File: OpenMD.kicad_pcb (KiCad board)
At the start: 4 copper layers, 90 x 55 mm, 189 parts, among them IC1 MP9485GN-Z, J1 GND, J2 Digital, J3 Analog, J4 Sensors, J5 A, J6 B, J7 C, J8 V_{BATT}, Q1 EPC2088, Q2 EPC2088, Q3 EPC2088, Q7 EPC2088, Q8 EPC2088, Q9 EPC2088, U1 UP1966E, U10 INA241A2xDDF, U2 UP1966E, U3 UP1966E, U7 ADA4610-4xCP, U8 INA241A2xDDF, U9 INA241A2xDDF

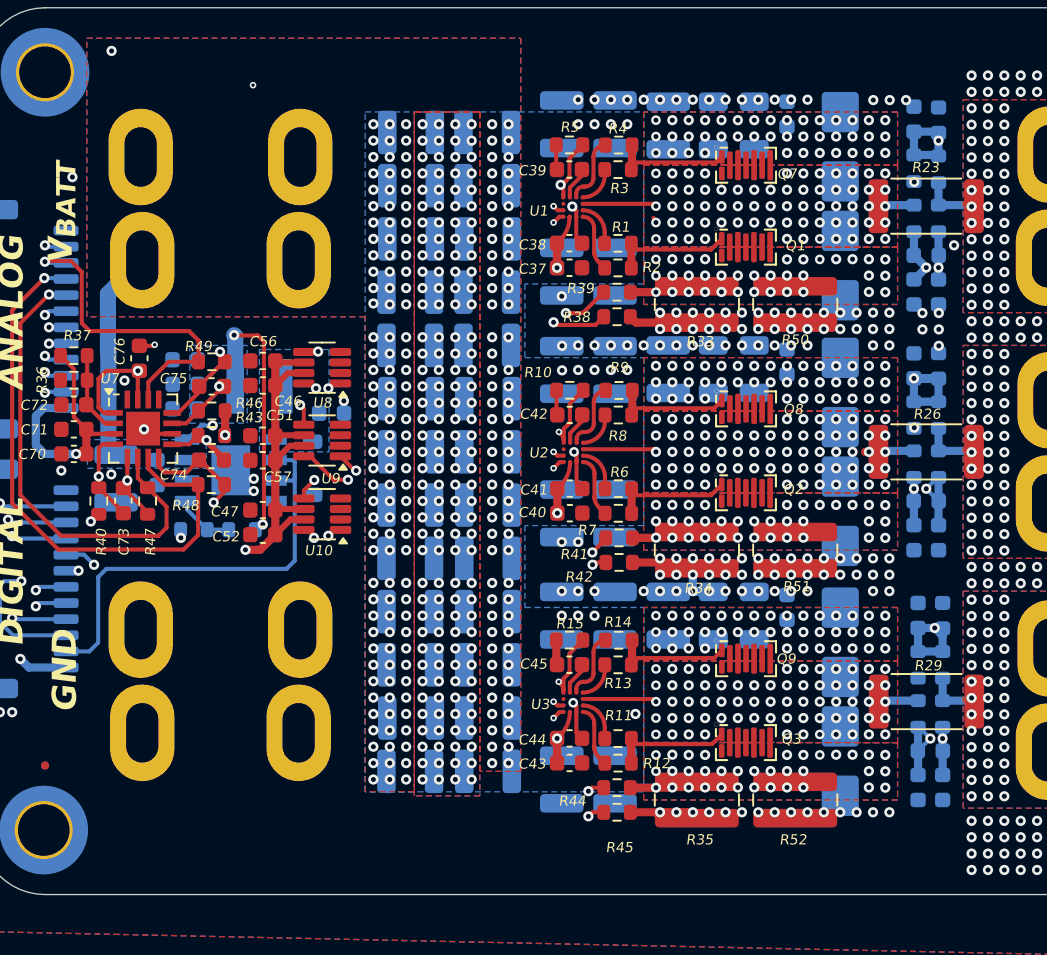
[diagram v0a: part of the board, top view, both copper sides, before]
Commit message: added license and almost ready for prod
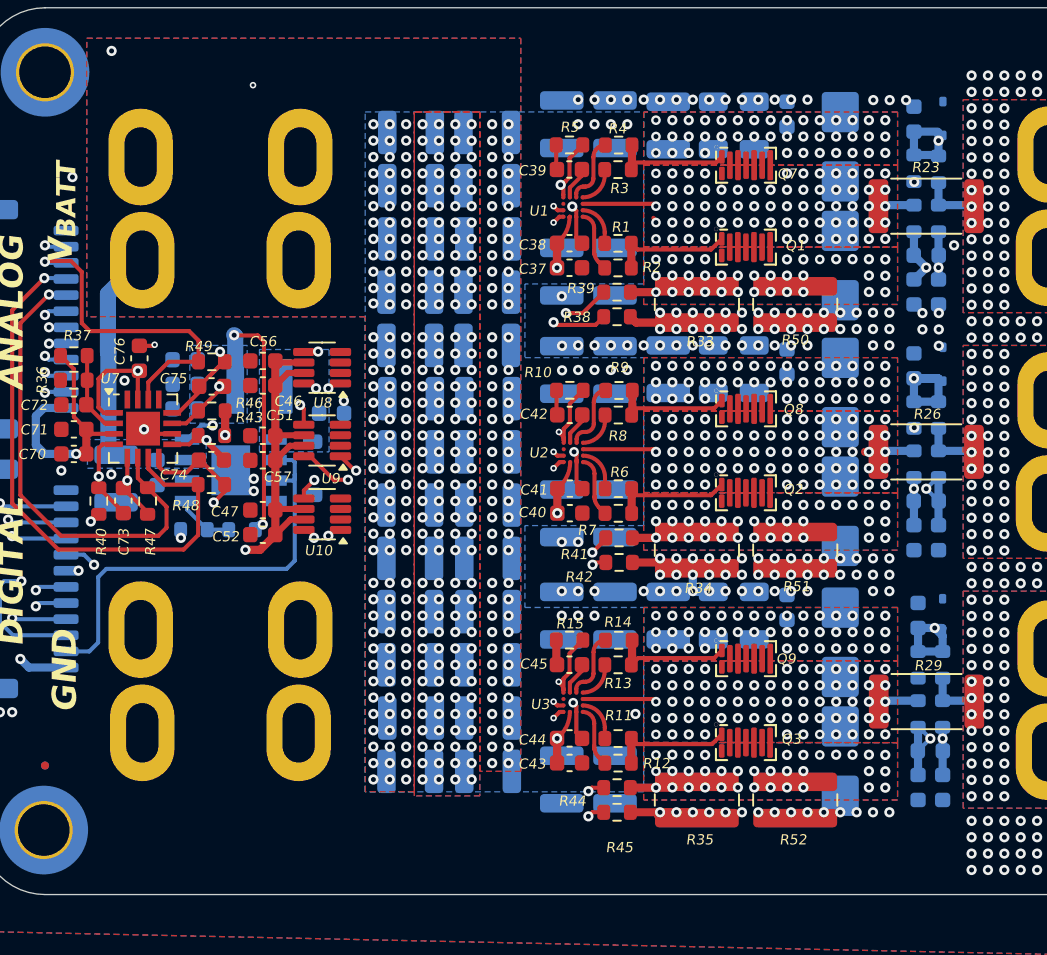
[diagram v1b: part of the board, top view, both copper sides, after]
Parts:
- removed REF**: ESD-Logo_6.6x6mm_SilkScreen, Symbol:ESD-Logo_6.6x6mm_SilkScreen
- removed REF**: OSHW-Symbol_6.7x6mm_SilkScreen, Symbol:OSHW-Symbol_6.7x6mm_SilkScreen
- removed REF**: WEEE-Logo_4.2x6mm_SilkScreen, Symbol:WEEE-Logo_4.2x6mm_SilkScreen
- D10: value D_Schottky -> 1V
- D7, D8, D9: footprint Diode_SMD:D_0603_1608Metric -> Diode_SMD:D_SOD-323
- moved D7 0.29 mm to (152.8, 82.2)
- moved D8 0.29 mm to (152.8, 97.4)

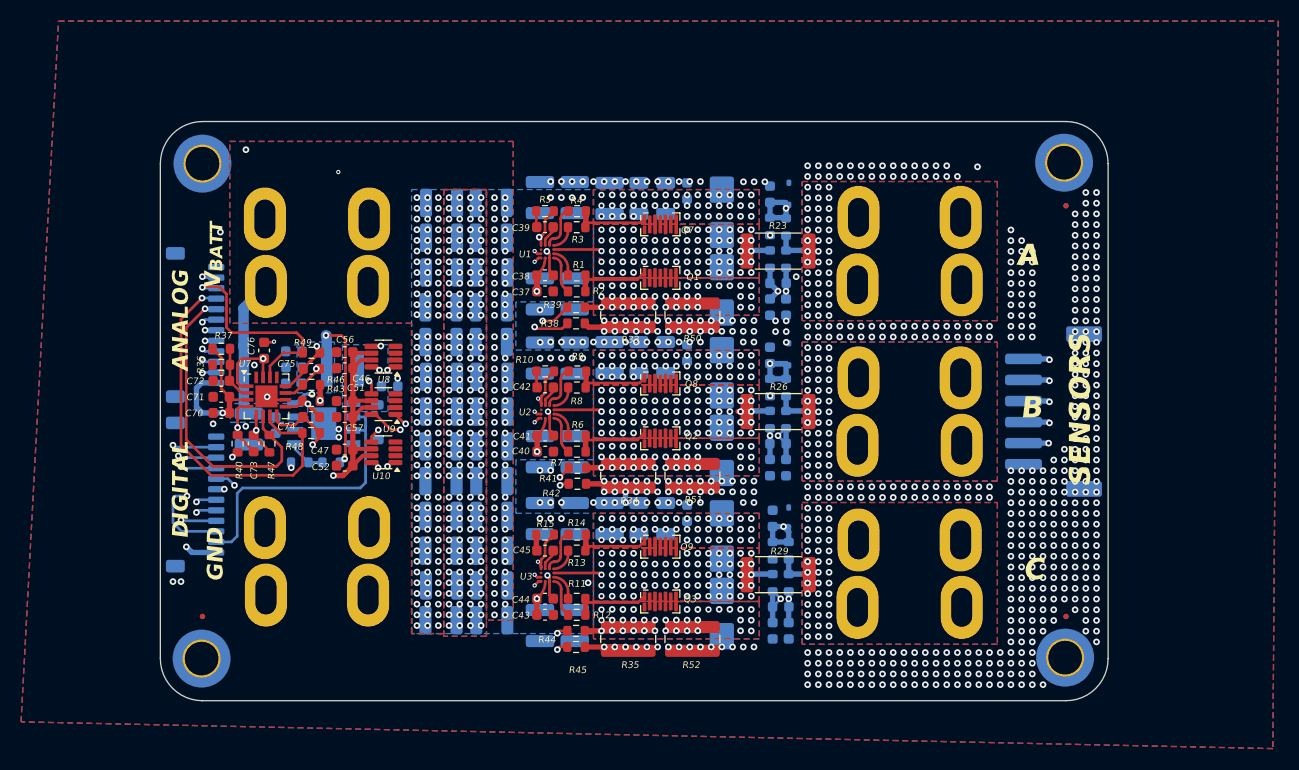
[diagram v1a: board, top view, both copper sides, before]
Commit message: first fab run
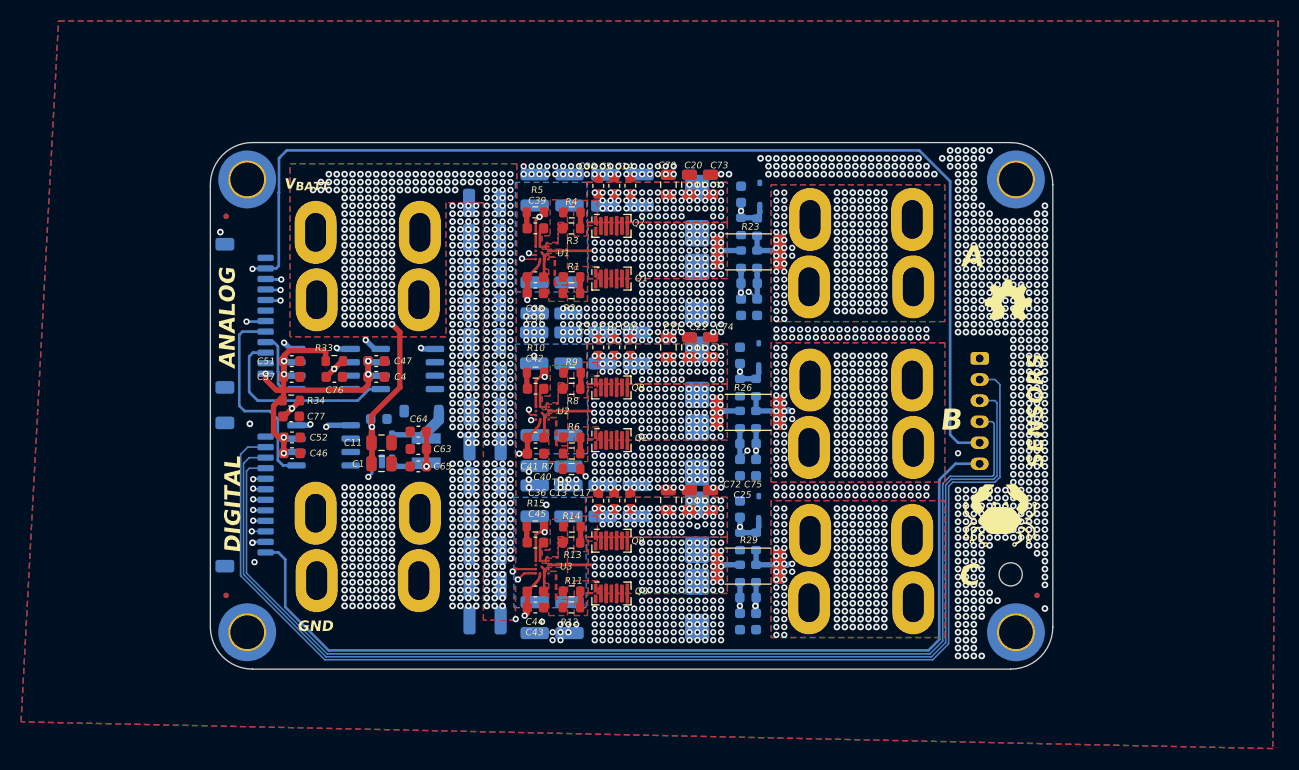
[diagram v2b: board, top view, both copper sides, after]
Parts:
- removed C56: 4.7uF, Capacitor_SMD:C_0603_1608Metric
- removed C61, C83, C84, C85: 10uF, Capacitor_SMD:C_1210_3225Metric
- removed C66: 100nF, Capacitor_SMD:C_0603_1608Metric
- removed the G*** at (139.1, 105.6)
- removed IC1: MP9485GN-Z, OpenMD:SOIC127P600X170-9N
- removed R31, R32: 240k, Resistor_SMD:R_0603_1608Metric
- removed R35, R50, R51, R52: .5m, Resistor_SMD:R_1020_2550Metric
- removed R36, R37, R40, R43, R46, R47, R48, R49: 20k, Resistor_SMD:R_0603_1608Metric
- removed R38, R39, R41, R42, R44, R45: 1k, Resistor_SMD:R_0603_1608Metric
- removed U7: ADA4610-4xCP, Package_CSP:LFCSP-16-1EP_4x4mm_P0.65mm_EP2.1x2.1mm
- added G***: LOGO, OpenMD:CrabLabs, F.Cu at (172.9, 112.7)
- added G***: LOGO, OpenMD:CrabLabs, B.Cu at (172.9, 88.1)
- added H6: M2, MountingHole:MountingHole_2.2mm_M2, F.Cu at (173.9, 118.3)
- added IC2: RAA2118054GP3#JA0, Package_TO_SOT_SMD:SOT-23-5, B.Cu at (114.2, 106.5)
- added SYM1: Logo_Open_Hardware_Large, Symbol:OSHW-Symbol_8.9x8mm_SilkScreen, F.Cu at (173.6, 92.3)
- added SYM1: Logo_Open_Hardware_Large, Symbol:OSHW-Symbol_8.9x8mm_SilkScreen, B.Cu at (173.6, 113.8)
- added TH1: 10k, Resistor_SMD:R_0603_1608Metric, F.Cu at (132.2, 108.3)
- C1, C11, C20, C22, C25: value 10uF -> 1uF; footprint Capacitor_SMD:C_1210_3225Metric -> Capacitor_SMD:C_0805_2012Metric; moved to F.Cu
- C10, C13, C14, C16, C17, C5, C77: value 10uF -> 100nF; footprint Capacitor_SMD:C_1210_3225Metric -> Capacitor_SMD:C_0603_1608Metric; moved to F.Cu
- C12, C15, C18, C19, C2, C21, C23, C24, C26, C27, C3, C6, C7, C78, C79, C8, C80, C81, C82, C86, C87, C88, C89, C9, C91: value 10uF -> 4.7uF
- C28, C29, C31, C32, C34, C35: footprint Capacitor_SMD:C_1206_3216Metric -> Capacitor_SMD:C_1210_3225Metric
- C30, C33, C36, C63, C64, C65: moved to F.Cu
- C4: value 10uF -> 4.7uF; footprint Capacitor_SMD:C_1210_3225Metric -> Capacitor_SMD:C_0603_1608Metric; moved to F.Cu
- C70: value 100nF -> 1uF; footprint Capacitor_SMD:C_0603_1608Metric -> Capacitor_SMD:C_0805_2012Metric
- C71: value 4.7uF -> 1uF; footprint Capacitor_SMD:C_0603_1608Metric -> Capacitor_SMD:C_0805_2012Metric
- C72, C73, C74, C75: value 10nF -> 1uF; footprint Capacitor_SMD:C_0603_1608Metric -> Capacitor_SMD:C_0805_2012Metric
- D1, D2, D3, D4, D5, D6: value S3BB-13-F -> .85V
- D10: value 1V -> .85V
- D7, D8, D9: value 3.7V -> 3.3V
- H1, H2, H3, H4: value MountingHole_Pad -> M3
- J4: footprint Connector_JST:JST_PH_S6B-PH-SM4-TB_1x06-1MP_P2.00mm_Horizontal -> Connector_JST:JST_PH_S6B-PH-K_1x06_P2.00mm_Horizontal
- L1: value 33uH -> 22uH; footprint Inductor_SMD:L_Abracon_ASPI-4030S -> Inductor_SMD:L_Abracon_ASPI-3012S
- Q1, Q2, Q3, Q7, Q8, Q9: value EPC2088 -> EPC2065
- R1, R11, R14, R4, R6, R9: value 0 -> 1
- R33, R34: value .5m -> 10k; footprint Resistor_SMD:R_1020_2550Metric -> Resistor_SMD:R_0603_1608Metric
- U10, U8, U9: value INA241A2xDDF -> INA240A2; footprint Package_TO_SOT_SMD:SOT-23-8 -> Package_SO:SO-8_3.9x4.9mm_P1.27mm; moved to B.Cu
- moved FID2 79.8 mm to (99.4, 84.3)
- moved FID6 79.8 mm to (99.4, 84.3)
- moved C73 49.9 mm to (145.4, 81.3)
- moved C70 47.7 mm to (141.4, 81.3), turned to 90 degrees
- moved C20 47.6 mm to (143.4, 81.3), turned to 90 degrees
- moved C72 43.9 mm to (141.4, 111.3), turned to 90 degrees
- moved C71 42.7 mm to (141.4, 96.8), turned to 90 degrees
- moved C75 39.9 mm to (145.4, 111.3), turned to 90 degrees
- moved C74 38.5 mm to (145.4, 96.8), turned to 90 degrees
- moved C14 33.3 mm to (137.8, 81.4), turned to 90 degrees
- moved R34 32.8 mm to (105.6, 101.8), turned to 0 degrees
- moved C11 31.7 mm to (114.1, 105.8), turned to 0 degrees
- moved C22 28.5 mm to (143.4, 96.8), turned to 90 degrees
- moved R33 28.2 mm to (109.7, 98.1), turned to 0 degrees
- moved C13 27.2 mm to (136.3, 111.3), turned to 90 degrees
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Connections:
- C4 pad 1: /V_{BATT} -> /V_{ANA}
- C70 pad 1: /V_{ANA} -> /V_{BATT}
- C71 pad 1: /V_{ANA} -> /V_{BATT}
- C72 pad 1: Net-(U7A-+) -> /V_{BATT}
- C73 pad 1: Net-(U7B-+) -> /V_{BATT}
- C73 pad 2: Net-(U7B--) -> /GND
- C74 pad 1: Net-(U7C-+) -> /V_{BATT}
- C74 pad 2: Net-(U7C--) -> /GND
- C75 pad 1: Net-(U7D-+) -> /V_{BATT}
- C75 pad 2: Net-(U7D--) -> /GND
- C76 pad 1: /Driver Current Sensors/V_{REF} -> /M_TEMP_SENSE
- C77 pad 1: /V_{BATT} -> /DRV_TEMP_SENSE
- J3 pad 10: /DRV_I_SENSE.C -> /V_SENSE.C
- J3 pad 2: /I_SENSE.A -> /GND
- J3 pad 3: /I_SENSE.B -> /I_SENSE.A
- J3 pad 4: /I_SENSE.C -> /I_SENSE.B
- J3 pad 5: /V_SENSE.A -> /I_SENSE.C
- J3 pad 6: /V_SENSE.B -> /DRV_TEMP_SENSE
- J3 pad 7: /V_SENSE.C -> /GND
- J3 pad 8: /DRV_I_SENSE.A -> /V_SENSE.A
- J3 pad 9: /DRV_I_SENSE.B -> /V_SENSE.B
- J4 pad 1: /V_{DIG} -> /GND
- J4 pad 2: /M_TEMP_SENSE -> /HALL.C
- J4 pad 3: /HALL.A -> /HALL.B
- J4 pad 4: /HALL.B -> /HALL.A
- J4 pad 5: /HALL.C -> /M_TEMP_SENSE
- J4 pad 6: /GND -> /V_{DIG}
- Q1 pad 2: /DRV_CURR_SENSE.A -> /GND
- Q1 pad 4: /DRV_CURR_SENSE.A -> /GND
- Q1 pad 6: /DRV_CURR_SENSE.A -> /GND
- Q1 pad 8: /DRV_CURR_SENSE.A -> /GND
- Q2 pad 2: /DRV_CURR_SENSE.B -> /GND
- Q2 pad 4: /DRV_CURR_SENSE.B -> /GND
- Q2 pad 6: /DRV_CURR_SENSE.B -> /GND
- Q2 pad 8: /DRV_CURR_SENSE.B -> /GND
- Q3 pad 2: /DRV_CURR_SENSE.C -> /GND
- Q3 pad 4: /DRV_CURR_SENSE.C -> /GND
- Q3 pad 6: /DRV_CURR_SENSE.C -> /GND
- Q3 pad 8: /DRV_CURR_SENSE.C -> /GND
- R33 pad 1: /DRV_CURR_SENSE.A -> /V_{ANA}
- R33 pad 2: /GND -> /M_TEMP_SENSE
- R34 pad 1: /DRV_CURR_SENSE.B -> /V_{ANA}
- R34 pad 2: /GND -> /DRV_TEMP_SENSE
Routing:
- net /DRV_TEMP_SENSE: track 0.00 -> 86.1 mm, vias 0 -> 3
- net Net-(U7D--): track 76.0 -> 0.00 mm, vias 2 -> 0
- net Net-(U7D-+): track 74.8 -> 0.00 mm, vias 2 -> 0
- net /V_{DIG}: track 137.0 -> 90.5 mm, vias 2 -> 0
- net Net-(U7B-+): track 44.5 -> 0.00 mm, vias 2 -> 0
- net Net-(U7B--): track 42.7 -> 0.00 mm, vias 2 -> 0
- net /Phase Current Sensors/Current Sense A/V+: track 119.6 -> 81.9 mm
- net Net-(U7C-+): track 37.6 -> 0.00 mm, vias 2 -> 0
- net /DRV_I_SENSE.B: track 36.4 -> 0.00 mm, vias 1 -> 0
- net Net-(U7C--): track 35.1 -> 0.00 mm, vias 2 -> 0
- net /Phase Current Sensors/Current Sense A/V-: track 122.1 -> 89.8 mm
- net /Driver Current Sensors/V_{REF}: track 30.3 -> 0.00 mm, vias 3 -> 0
- net /DRV_I_SENSE.A: track 29.6 -> 0.00 mm, vias 1 -> 0
- net /HALL.A: track 134.9 -> 107.9 mm, vias 2 -> 0
- net /HALL.B: track 137.6 -> 112.2 mm, vias 2 -> 0
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- added copper zone on F.Cu, net /AH
- added copper zone on F.Cu, net /AL
- added copper zone on F.Cu, net /BH
- added copper zone on F.Cu, net /BL
- added copper zone on F.Cu, net /CH
- added copper zone on F.Cu, net /CL
- added copper zone on F.Cu, net /Predrivers/Gate Driver A/LGH
- added copper zone on F.Cu, net /Predrivers/Gate Driver A/LGL
- added copper zone on F.Cu, net /Predrivers/Gate Driver A/UGH
- added copper zone on F.Cu, net /Predrivers/Gate Driver A/UGL
- added copper zone on F.Cu, net /Predrivers/Gate Driver B/LGH
- added copper zone on F.Cu, net /Predrivers/Gate Driver B/LGL
- added copper zone on F.Cu, net /Predrivers/Gate Driver B/UGH
- added copper zone on F.Cu, net /Predrivers/Gate Driver B/UGL
- added copper zone on F.Cu, net /Predrivers/Gate Driver C/LGH
- added copper zone on F.Cu, net /Predrivers/Gate Driver C/LGL
- added copper zone on F.Cu, net /Predrivers/Gate Driver C/UGH
- added copper zone on F.Cu, net /Predrivers/Gate Driver C/UGL
- removed copper zone on B.Cu, net /DRV_CURR_SENSE.A
- removed copper zone on F.Cu, net /DRV_CURR_SENSE.A
- removed copper zone on In1.Cu, net /DRV_CURR_SENSE.A
- removed copper zone on In2.Cu, net /DRV_CURR_SENSE.A
- removed copper zone on B.Cu, net /DRV_CURR_SENSE.B
- removed copper zone on F.Cu, net /DRV_CURR_SENSE.B
- removed copper zone on In1.Cu, net /DRV_CURR_SENSE.B
- removed copper zone on In2.Cu, net /DRV_CURR_SENSE.B
- removed copper zone on B.Cu, net /DRV_CURR_SENSE.C
- removed copper zone on F.Cu, net /DRV_CURR_SENSE.C
- removed copper zone on In1.Cu, net /DRV_CURR_SENSE.C
- removed copper zone on In2.Cu, net /DRV_CURR_SENSE.C
- removed copper zone on B.Cu, net /Predriver Voltage Supply/SW
- removed copper zone on B.Cu, net /V_{DRV}
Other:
- board size 90 x 55 mm -> 80 x 50 mm
- board text removed: "OpenMD V0.1"
